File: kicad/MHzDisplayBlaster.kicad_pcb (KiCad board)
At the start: 2 copper layers, 50 x 39 mm, 7 parts, among them J1 Conn_02x15 DigitLHS, J2 Conn_02x15 DigitRHS, J3 Conn_01x03_Pin, U1 DC56-11GWA, U2 74LS04

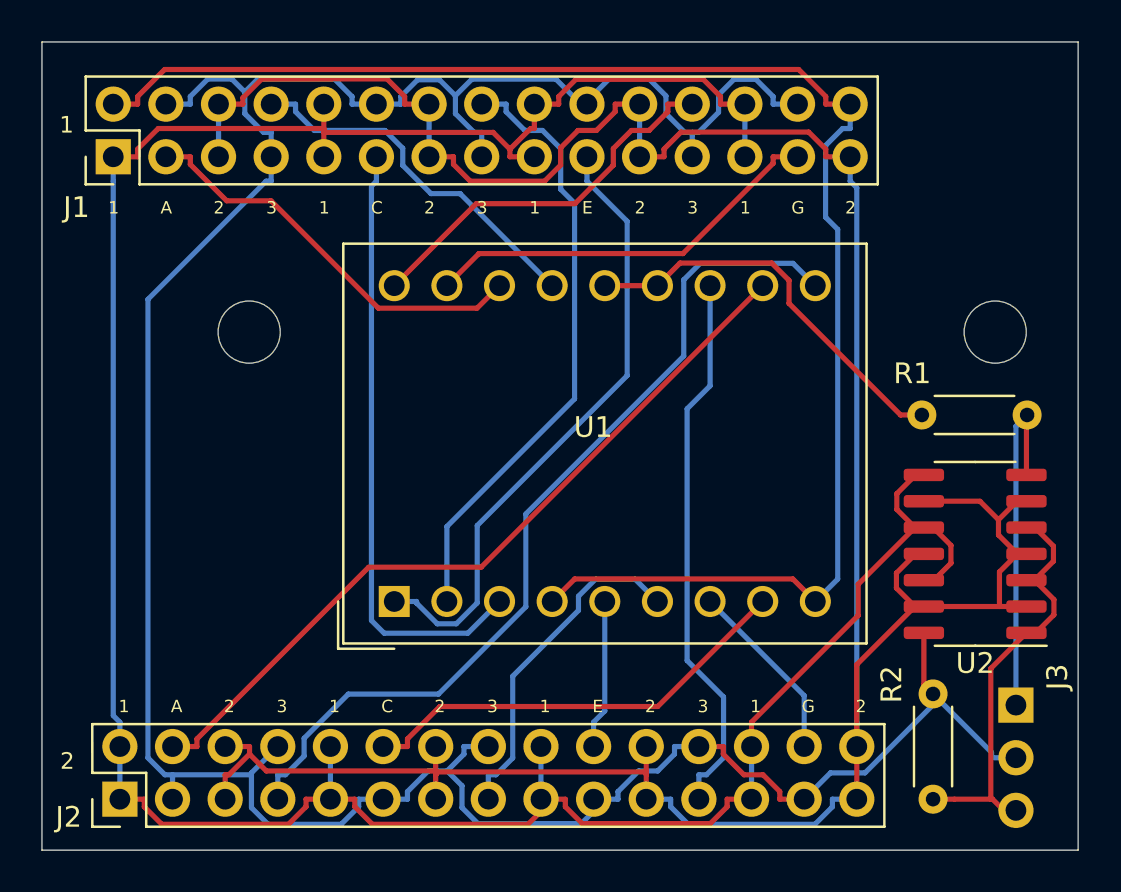
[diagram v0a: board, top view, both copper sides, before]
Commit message: Major Refactor and Cleanup
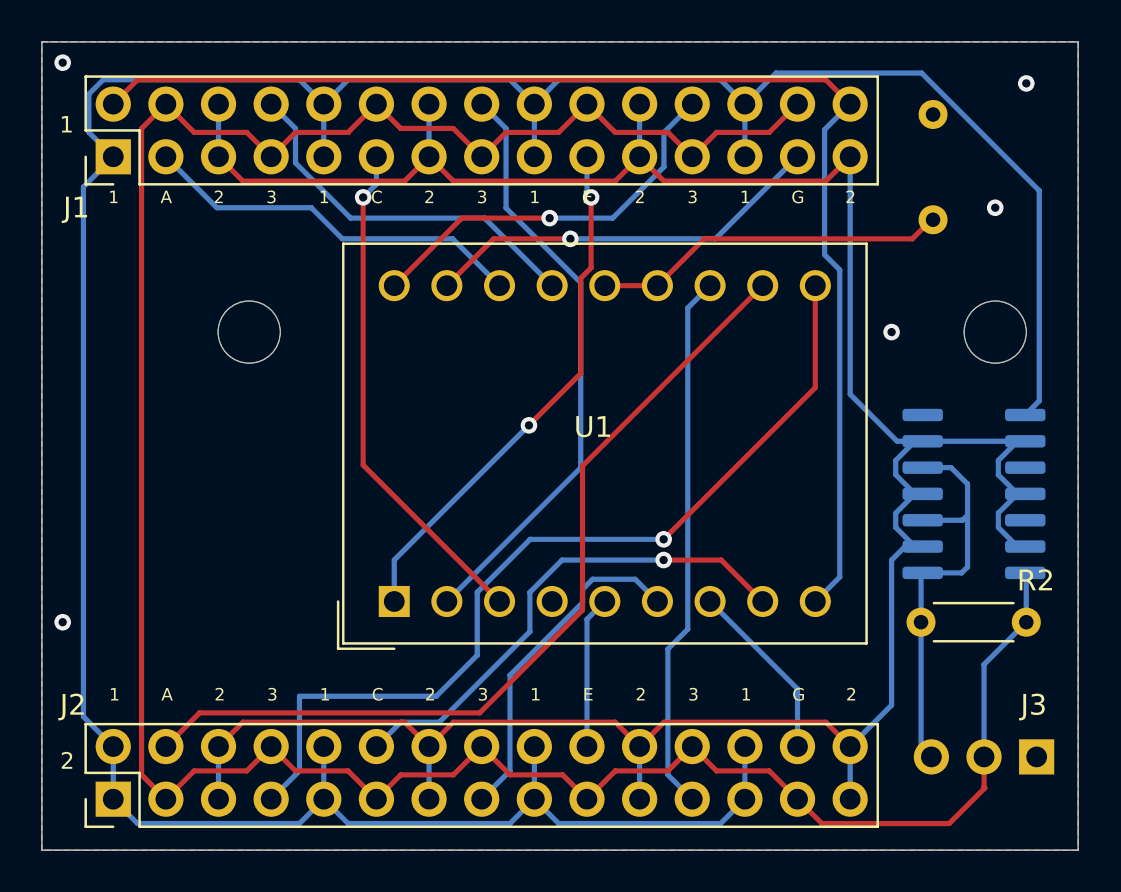
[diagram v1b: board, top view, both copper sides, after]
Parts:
- R1, U2: moved to B.Cu
- moved R1 15.2 mm to (143.0, 43.5), turned to -90 degrees
- moved R2 5.68 mm to (147.5, 68.0), turned to 180 degrees
- moved U2 2.89 mm to (145.0, 61.8), turned to 0 degrees
- moved J3 2.69 mm to (148.0, 74.5), turned to 90 degrees
- moved J2 0.32 mm to (103.4, 76.5)
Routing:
- net GND: track 17.1 -> 0.00 mm, vias 0 -> 5
- net DP: track 76.4 -> 61.8 mm
- net 3: track 143.2 -> 129.6 mm
- net 2: track 143.5 -> 132.5 mm
- net 1: track 137.2 -> 147.0 mm
- net DIG1_C: track 29.5 -> 24.5 mm, vias 0 -> 1
- net DIG1_E: track 30.2 -> 25.5 mm, vias 0 -> 2
- net DIG2_A: track 37.9 -> 42.1 mm
- net DIG2_C: track 21.4 -> 24.3 mm, vias 0 -> 1
- net DIG1_CC: track 19.4 -> 17.3 mm
- net DIG1_A: track 19.8 -> 18.7 mm
- net DIG1_D: track 29.6 -> 28.7 mm
- net Turbo: track 20.8 -> 20.2 mm
- net DIG2_F: track 26.7 -> 26.1 mm
- net DIG1_F: track 18.7 -> 19.0 mm, vias 0 -> 1
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- added copper zone on B.Cu, net GND
- added copper zone on F.Cu, net GND
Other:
- board text added: "Trb"
- board text removed: "Trbo"
